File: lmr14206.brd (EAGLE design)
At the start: 16.2 x 27.9 mm, 12 parts

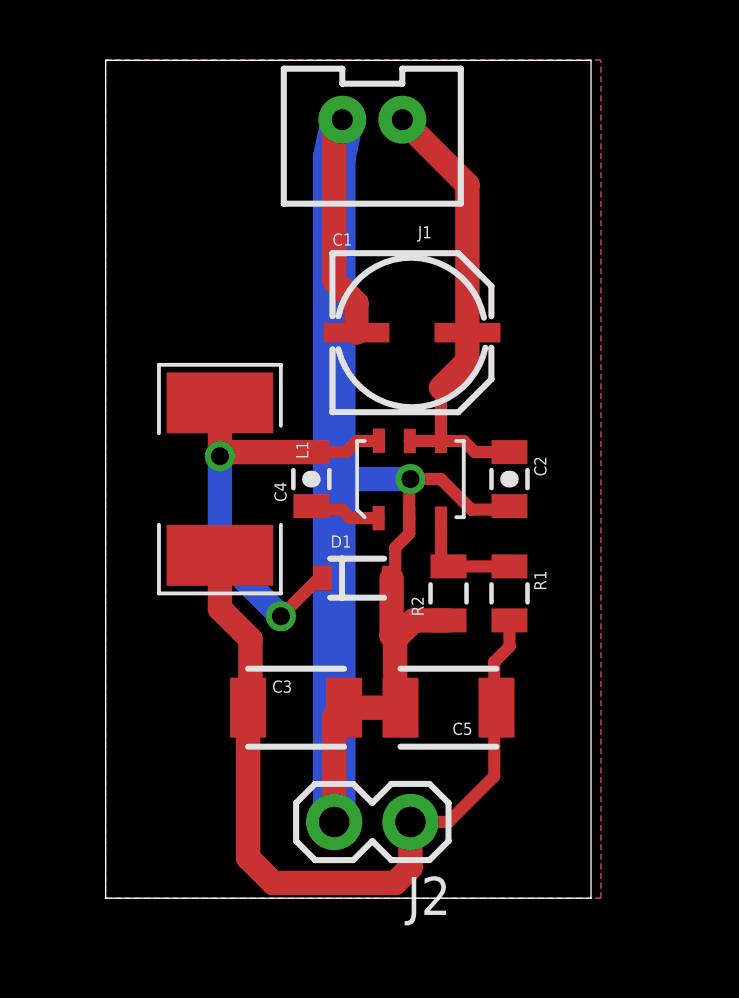
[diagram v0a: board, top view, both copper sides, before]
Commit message: Breakout board updates
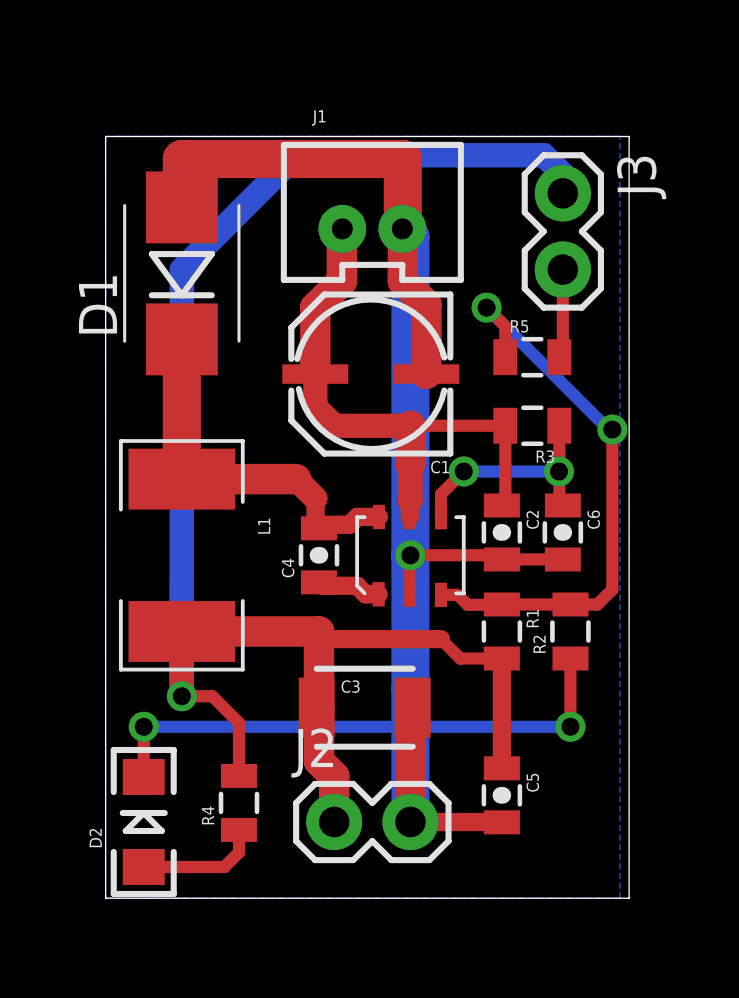
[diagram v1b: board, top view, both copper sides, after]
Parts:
- added C6: 1uF, SparkFun-Capacitors:0805-CAP
- added D2: YELLOW, SparkFun-LED:LED-1206
- added J3: (no value), SparkFun-Connectors:1X02
- added R3: 270k, SparkFun-Resistors:0805
- added R4: 680, SparkFun-Resistors:0805
- added R5: 34k, SparkFun-Resistors:0805
- C5: device SparkFun-Capacitors:1210 -> SparkFun-Capacitors:0805-CAP
- D1: value BAT20J -> (none); device SparkFun-DiscreteSemi:SOD-323 -> SparkFun-DiscreteSemi:SMB-DIODE
- moved D1 11.7 mm to (2.54, 20.8), turned to 90 degrees
- moved R2 4.26 mm to (15.5, 8.89)
- moved C5 3.42 mm to (13.2, 3.43), turned to 270 degrees
- moved L1 2.84 mm to (2.54, 11.4)
- moved C4 2.55 mm to (7.11, 11.4)
- moved U$1 2.54 mm to (10.2, 11.4)
- moved J2 2.54 mm to (7.62, 2.54), turned to 0 degrees
- moved J1 2.54 mm to (8.89, 22.9), turned to 0 degrees
- moved C3 2.29 mm to (8.64, 6.35)
- moved C1 2.18 mm to (8.89, 17.3), turned to 180 degrees
- moved C2 1.80 mm to (13.2, 12.2)
- moved R1 1.30 mm to (13.2, 8.89)
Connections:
- removed net 5V: C3.1, C5.1, J2.1, L1.P$2, R1.2
- new net FB: R1.1, R2.2, R5.1, U$1.3
- new net N$2: D2.A, R4.1
- new net N$5: C6.1, R3.1, U$1.4
- new net VCC: C3.1, C5.1, J2.1, J3.1, L1.P$2, R1.2, R4.2
- net GND: now also C6.2, D2.C
- net N$1: now also J3.2, R5.2; no longer R1.1, R2.2, U$1.3
- net VIN: now also R3.2; no longer U$1.4
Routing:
- net VCC: track 0.00 -> 60.7 mm, vias 0 -> 1
- net 5V: track 26.9 -> 0.00 mm
- net FB: track 0.00 -> 19.2 mm, vias 0 -> 2
- net GND: track 52.9 -> 69.1 mm, vias 1 -> 3
- net N$5: track 0.00 -> 7.89 mm, vias 0 -> 2
- net N$2: track 0.00 -> 4.13 mm
- net VIN: track 15.5 -> 18.7 mm
- net N$4: track 15.4 -> 12.6 mm, vias 2 -> 0
- net N$1: track 3.73 -> 2.97 mm
- removed copper zone on layer 1, net GND
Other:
- board size 16.2 x 27.9 mm -> 17.4 x 25.4 mm
